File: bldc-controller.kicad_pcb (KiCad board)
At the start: 2 copper layers, 56 x 39 mm, 57 parts, among them IC1 L6205PD, P1 CON_LED, P2 CON_LIDAR, P3 CON_MOTOR, P4 USB_OTG, P5 CON_SWD, P6 CON_HALL, P7 CON_PWR_BRD, U1 STM32F405R, U5 MPU6000, U7 LD1117S33TR, Y1 Crystal

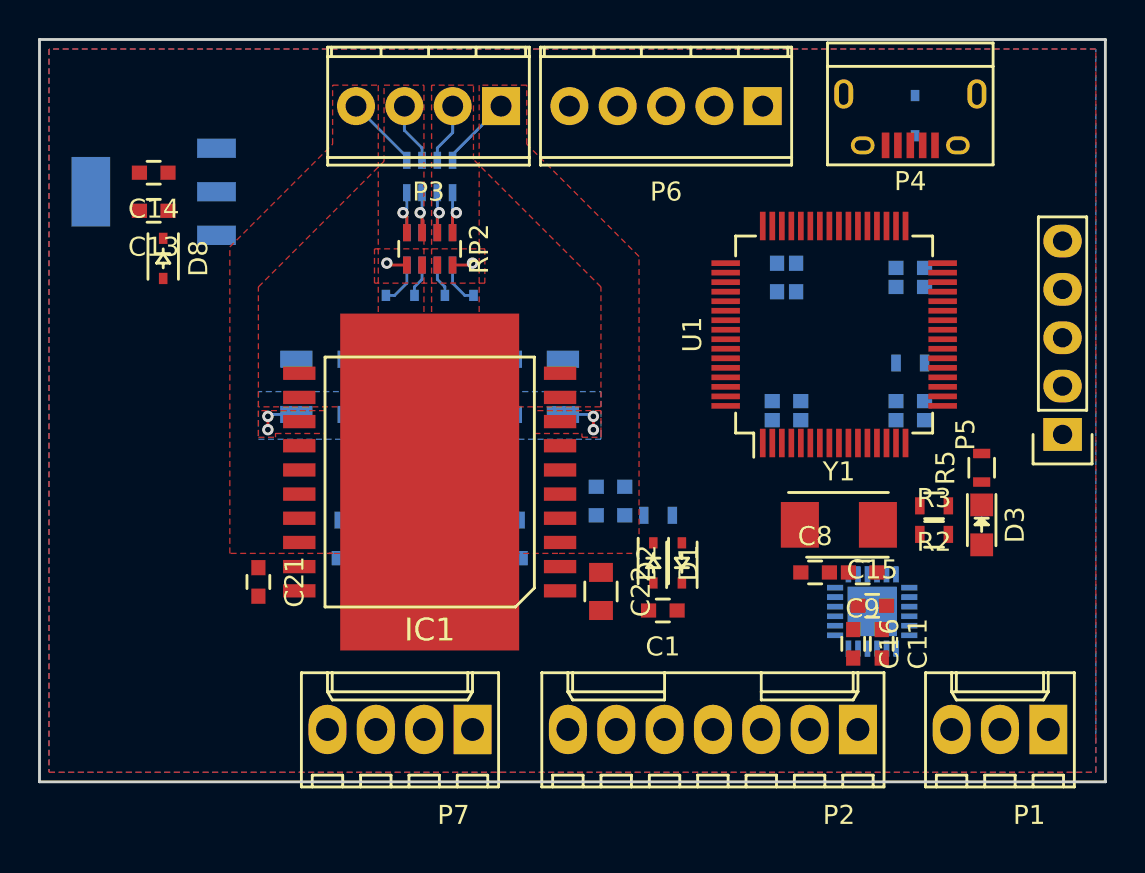
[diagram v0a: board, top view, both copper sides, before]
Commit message: routed
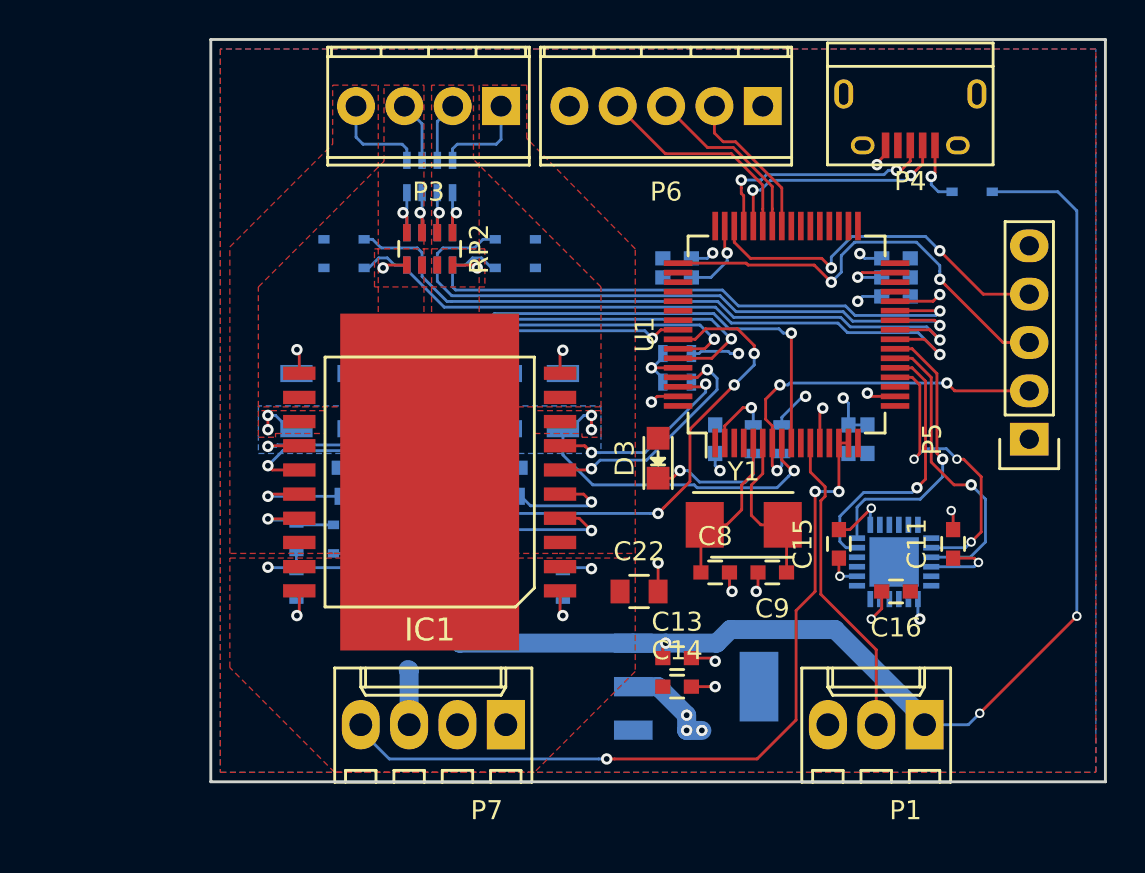
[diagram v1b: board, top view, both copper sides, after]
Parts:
- removed P2: CON_LIDAR, Connectors_Molex:Molex_KK-6410-07_07x2.54mm_Straight
- C1, C21, D1, D2, D8, R2, R3, R5: moved to B.Cu
- moved U7 38.6 mm to (149.5, 100.0), turned to 90 degrees
- moved C14 38.5 mm to (148.5, 100.0), turned to 0 degrees
- moved C13 36.2 mm to (148.5, 98.5), turned to 0 degrees
- moved D8 24.2 mm to (134.4, 98.0)
- moved C1 19.7 mm to (128.5, 92.0), turned to 270 degrees
- moved D2 17.4 mm to (131.5, 91.5), turned to 0 degrees
- moved D3 17.4 mm to (147.5, 88.0), turned to 90 degrees
- moved D1 15.8 mm to (131.5, 93.0), turned to 0 degrees
- moved R2 15.7 mm to (148.5, 82.5)
- moved R3 15.7 mm to (148.5, 84.0)
- moved R1 13.1 mm to (134.5, 92.5), turned to 90 degrees
- moved R5 12.1 mm to (152.5, 87.0)
- moved C17 9.45 mm to (148.5, 78.5), turned to 180 degrees
- moved C2 9.12 mm to (136.0, 92.5), turned to 270 degrees
- moved R4 7.85 mm to (154.0, 87.0), turned to 270 degrees
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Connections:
- P4 pad 6: Net-(P4-Pad6) -> GND
- P7 pad 2: Net-(D8-Pad2) -> VPP
- P7 pad 3: /Power/RX_PWR_BOARD -> Net-(D8-Pad2)
- P7 pad 4: /Power/TX_PWR_BOARD -> /Power/RX_TX_PWR_BOARD
- U1 pad 14: /Power/RX_PWR_BOARD -> /Power/RX_TX_PWR_BOARD
- U1 pad 15: /Power/RX_PWR_BOARD -> /Power/RX_TX_PWR_BOARD
- U1 pad 16: /Power/TX_PWR_BOARD -> (no net)
- U1 pad 17: /Power/TX_PWR_BOARD -> (no net)
- U1 pad 37: /CON_LIDAR/LIDAR_TX -> (no net)
- U1 pad 38: /CON_LIDAR/LIDAR_RX -> (no net)
- U1 pad 39: /CON_LIDAR/LIDAR_MOTOR_EN -> (no net)
- U1 pad 56: /driver/EN_A -> /driver/EN_B
- U1 pad 57: /driver/EN_B -> /driver/EN_A
- U1 pad 58: /driver/IN1_A -> /driver/IN2_B
- U1 pad 59: /driver/IN2_A -> /driver/IN1_B
- U1 pad 61: /driver/IN1_B -> /driver/IN1_A
- U1 pad 62: /driver/IN2_B -> /driver/IN2_A
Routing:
- net +5V: track 0.00 -> 67.4 mm, vias 0 -> 3
- net /Power/RX_TX_PWR_BOARD: track 0.00 -> 41.4 mm, vias 0 -> 3
- net /CUR_SENSE_4/OUT_2: track 1.76 -> 35.8 mm, vias 0 -> 1
- net /CUR_SENSE_4/OUT_1: track 2.32 -> 35.4 mm, vias 0 -> 1
- net /CUR_SENSE_4/OUT_3: track 1.76 -> 34.6 mm, vias 0 -> 1
- net /driver/IN1_B: track 0.00 -> 32.4 mm, vias 0 -> 2
- net /driver/SENSE_B: track 2.22 -> 34.2 mm, vias 2 -> 3
- net /driver/IN2_B: track 0.00 -> 30.7 mm, vias 0 -> 2
- net /CUR_SENSE_4/OUT_4: track 2.32 -> 32.5 mm, vias 0 -> 1
- net GND: track 2.18 -> 28.5 mm, vias 2 -> 19
- net /driver/EN_A: track 0.00 -> 24.8 mm, vias 0 -> 3
- net /SWDIO/SWDCLK: track 0.00 -> 22.9 mm, vias 0 -> 2
- net /driver/EN_B: track 0.00 -> 21.2 mm, vias 0 -> 1
- net /SWDIO/NRST: track 0.00 -> 19.4 mm, vias 0 -> 3
- net /SWDIO/SWDIO: track 0.00 -> 19.2 mm, vias 0 -> 2
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- added copper zone on F.Cu, net VPP
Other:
- board size 56 x 39 mm -> 47 x 39 mm
